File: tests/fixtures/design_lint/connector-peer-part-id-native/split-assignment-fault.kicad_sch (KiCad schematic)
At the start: 2 parts, among them U1 Synthetic power module, U2 Synthetic power module

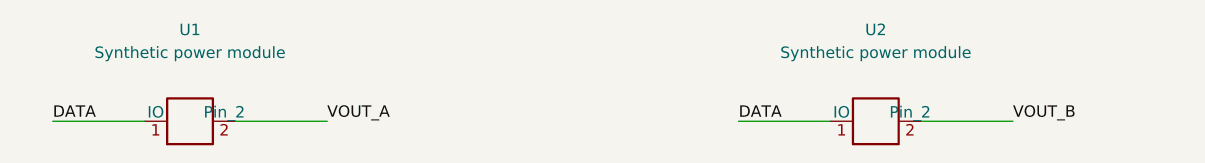
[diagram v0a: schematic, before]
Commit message: Add comparable peer pin lint gates
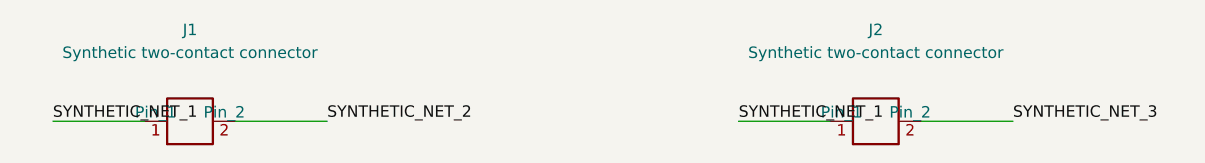
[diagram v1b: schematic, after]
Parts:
- J1: renamed from U1; value Synthetic power module -> Synthetic two-contact connector; footprint Synthetic:Module -> Synthetic:Connector_2x1; symbol Synthetic:PowerModule -> Synthetic:GenericPort; PART_ID SYNTHETIC-POWER-MODULE-001 -> SYNTHETIC-CONNECTOR-2PIN-001
- J2: renamed from U2; value Synthetic power module -> Synthetic two-contact connector; footprint Synthetic:Module -> Synthetic:Connector_2x1; symbol Synthetic:PowerModuleAlias -> Synthetic:GenericPortAlias; PART_ID SYNTHETIC-POWER-MODULE-001 -> SYNTHETIC-CONNECTOR-2PIN-001
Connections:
- net DATA renamed SYNTHETIC_NET_1
- net VOUT_A renamed SYNTHETIC_NET_2
- net VOUT_B renamed SYNTHETIC_NET_3
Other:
- title: Synthetic power-output peer control -> Synthetic PART_ID connector split-assignment fault
- moved on the sheet: J1, J2
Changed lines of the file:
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@@
 (kicad_sch (version 20231120) (generator "eeschema")
   (paper "A4")
-  (title_block (title "Synthetic power-output peer control")
+  (title_block (title "Synthetic PART_ID connector split-assignment fault")
     (comment 1 "NOT FOR MANUFACTURE - tooling fixture"))
-  (symbol (lib_id "Synthetic:PowerModule") (at 88.9 78.74 0) (unit 1)
+  (symbol (lib_id "Synthetic:GenericPort") (at 88.9 78.74 0) (unit 1)
     (in_bom yes) (on_board yes) (dnp no)
-    (property "Reference" "U1" (at 88.9 68.58 0) (effects (font (size 1.27 1.27))))
-    (property "Value" "Synthetic power module" (at 88.9 71.12 0) (effects (font (size 1.27 1.27))))
-    (property "Footprint" "Synthetic:Module" (at 88.9 78.74 0) (effects (font (size 1.27 1.27)) hide))
-    (property "PART_ID" "SYNTHETIC-POWER-MODULE-001" (at 88.9 78.74 0) (effects (font (size 1.27 1.27)) hide))
+    (property "Reference" "J1" (at 88.9 68.58 0) (effects (font (size 1.27 1.27))))
+    (property "Value" "Synthetic two-contact connector" (at 88.9 71.12 0) (effects (font (size 1.27 1.27))))
+    (property "Footprint" "Synthetic:Connector_2x1" (at 88.9 78.74 0) (effects (font (size 1.27 1.27)) hide))
+    (property "PART_ID" "SYNTHETIC-CONNECTOR-2PIN-001" (at 88.9 78.74 0) (effects (font (size 1.27 1.27)) hide))
     (property "Datasheet" "" (at 88.9 78.74 0) (effects (font (size 1.27 1.27)) hide))
     (pin "1")
     (pin "2")
-    (instances (project "Synthetic peer power-output fixture" (path "/58fe9fab-a929-4a44-a7fd-b83188082220" (reference "U1") (unit 1))))
+    (instances (project "Synthetic PART_ID connector pin fixture" (path "/58fe9fab-a929-4a44-a7fd-b83188082220" (reference "J1") (unit 1))))
   )
-  (symbol (lib_id "Synthetic:PowerModuleAlias") (at 165.1 78.74 0) (unit 1)
+  (symbol (lib_id "Synthetic:GenericPortAlias") (at 165.1 78.74 0) (unit 1)
     (in_bom yes) (on_board yes) (dnp no)
-    (property "Reference" "U2" (at 165.1 68.58 0) (effects (font (size 1.27 1.27))))
-    (property "Value" "Synthetic power module" (at 165.1 71.12 0) (effects (font (size 1.27 1.27))))
-    (property "Footprint" "Synthetic:Module" (at 165.1 78.74 0) (effects (font (size 1.27 1.27)) hide))
-    (property "PART_ID" "SYNTHETIC-POWER-MODULE-001" (at 165.1 78.74 0) (effects (font (size 1.27 1.27)) hide))
+    (property "Reference" "J2" (at 165.1 68.58 0) (effects (font (size 1.27 1.27))))
+    (property "Value" "Synthetic two-contact connector" (at 165.1 71.12 0) (effects (font (size 1.27 1.27))))
+    (property "Footprint" "Synthetic:Connector_2x1" (at 165.1 78.74 0) (effects (font (size 1.27 1.27)) hide))
+    (property "PART_ID" "SYNTHETIC-CONNECTOR-2PIN-001" (at 165.1 78.74 0) (effects (font (size 1.27 1.27)) hide))
     (property "Datasheet" "" (at 165.1 78.74 0) (effects (font (size 1.27 1.27)) hide))
     (pin "1")
     (pin "2")
-    (instances (project "Synthetic peer power-output fixture" (path "/58fe9fab-a929-4a44-a7fd-b83188082220" (reference "U2") (unit 1))))
+    (instances (project "Synthetic PART_ID connector pin fixture" (path "/58fe9fab-a929-4a44-a7fd-b83188082220" (reference "J2") (unit 1))))
   )
   (wire (pts (xy 83.82 78.74) (xy 73.66 78.74))
     (stroke (width 0) (type default))
 )
-  (label "DATA" (at 73.66 78.74 0)
+  (label "SYNTHETIC_NET_1" (at 73.66 78.74 0)
     (effects (font (size 1.27 1.27)) (justify left bottom))
 )
@@
     (stroke (width 0) (type default))
 )
-  (label "DATA" (at 149.86 78.74 0)
+  (label "SYNTHETIC_NET_1" (at 149.86 78.74 0)
     (effects (font (size 1.27 1.27)) (justify left bottom))
 )
@@
     (stroke (width 0) (type default))
 )
-  (label "VOUT_A" (at 104.14 78.74 0)
+  (label "SYNTHETIC_NET_2" (at 104.14 78.74 0)
     (effects (font (size 1.27 1.27)) (justify left bottom))
 )
@@
     (stroke (width 0) (type default))
 )
-  (label "VOUT_B" (at 180.34 78.74 0)
+  (label "SYNTHETIC_NET_3" (at 180.34 78.74 0)
     (effects (font (size 1.27 1.27)) (justify left bottom))
 )
